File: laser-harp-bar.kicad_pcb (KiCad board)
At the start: 2 copper layers, 170 x 32 mm, 20 parts, among them J1 TO_BASE, Q1 PT204-6C, Q2 PT204-6C, Q3 PT204-6C, Q4 PT204-6C, Q5 PT204-6C, Q6 PT204-6C, Q7 PT204-6C, Q8 PT204-6C

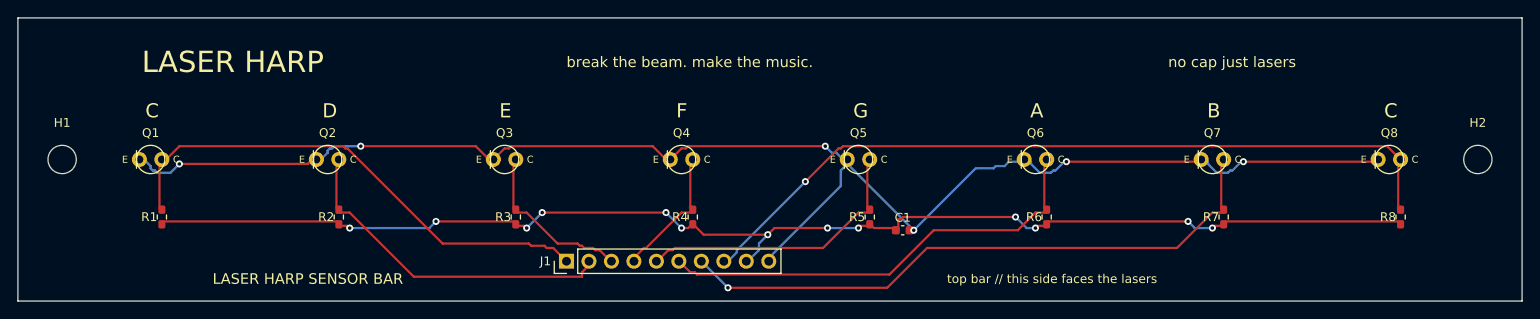
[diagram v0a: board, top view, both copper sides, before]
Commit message: added finishing touches
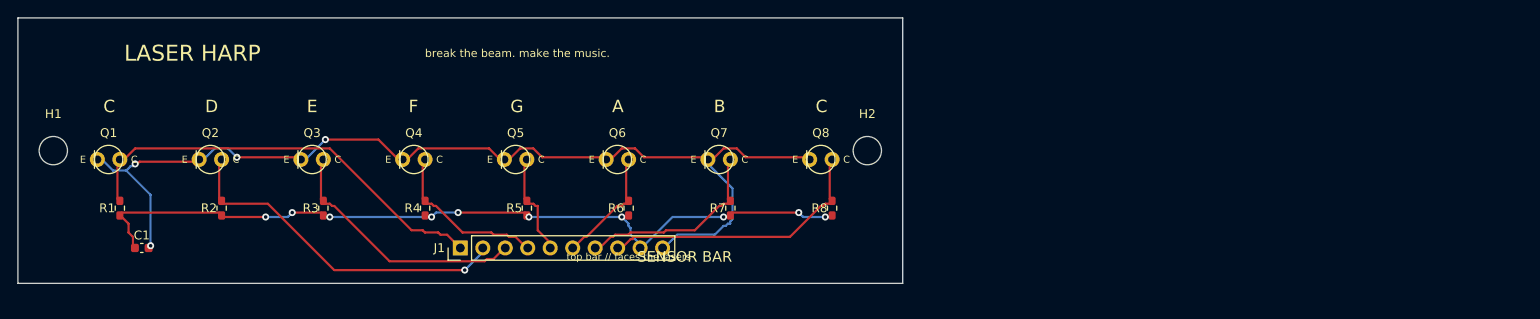
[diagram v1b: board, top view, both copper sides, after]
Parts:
- moved C1 86.0 mm to (14.0, 26.0)
- moved H2 69.0 mm to (96.0, 15.0)
- moved R8 64.3 mm to (92.0, 21.5)
- moved Q8 64.2 mm to (90.8, 16.0)
- moved R7 55.8 mm to (80.5, 21.5)
- moved Q7 55.8 mm to (79.2, 16.0)
- moved R6 47.3 mm to (69.0, 21.5)
- moved Q6 47.2 mm to (67.8, 16.0)
- moved R5 38.8 mm to (57.5, 21.5)
- moved Q5 38.8 mm to (56.2, 16.0)
- moved R4 30.3 mm to (46.0, 21.5)
- moved Q4 30.2 mm to (44.8, 16.0)
- moved R3 21.8 mm to (34.5, 21.5)
- moved Q3 21.8 mm to (33.2, 16.0)
- moved R2 13.3 mm to (23.0, 21.5)
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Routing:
- net /+3V3: track 144.4 -> 85.4 mm, vias 13 -> 10
- net /SENS8: track 85.8 -> 29.1 mm, vias 1 -> 0
- net /GND: track 157.0 -> 101.8 mm, vias 6 -> 4
- net /SENS7: track 67.6 -> 20.0 mm, vias 1 -> 0
- net /SENS6: track 48.8 -> 11.1 mm
- net /SENS5: track 30.1 -> 9.37 mm
- net /SENS3: track 16.8 -> 26.6 mm
- net /SENS1: track 54.6 -> 45.5 mm
- net /SENS4: track 12.7 -> 16.4 mm
- net /SENS2: track 36.2 -> 36.6 mm, vias 0 -> 1
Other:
- board size 170 x 32 mm -> 100 x 30 mm
- board text added: "SENSOR BAR"
- board text added: "top bar // faces the lasers"
- board text removed: "LASER HARP SENSOR BAR"
- board text removed: "no cap just lasers"
- board text removed: "top bar // this side faces the lasers"
